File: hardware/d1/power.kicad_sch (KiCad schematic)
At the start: 46 parts, among them U10 BLM15PX601SN1D, U11 TPS7A2033PDBVR, U12 TPS7A2018PDBVR, U13 TPS7A2018PDBVR, U7 TPS7A2018PDBVR, U8 TPS7A2033PDBVR, U9 TPS560430XFDBVR

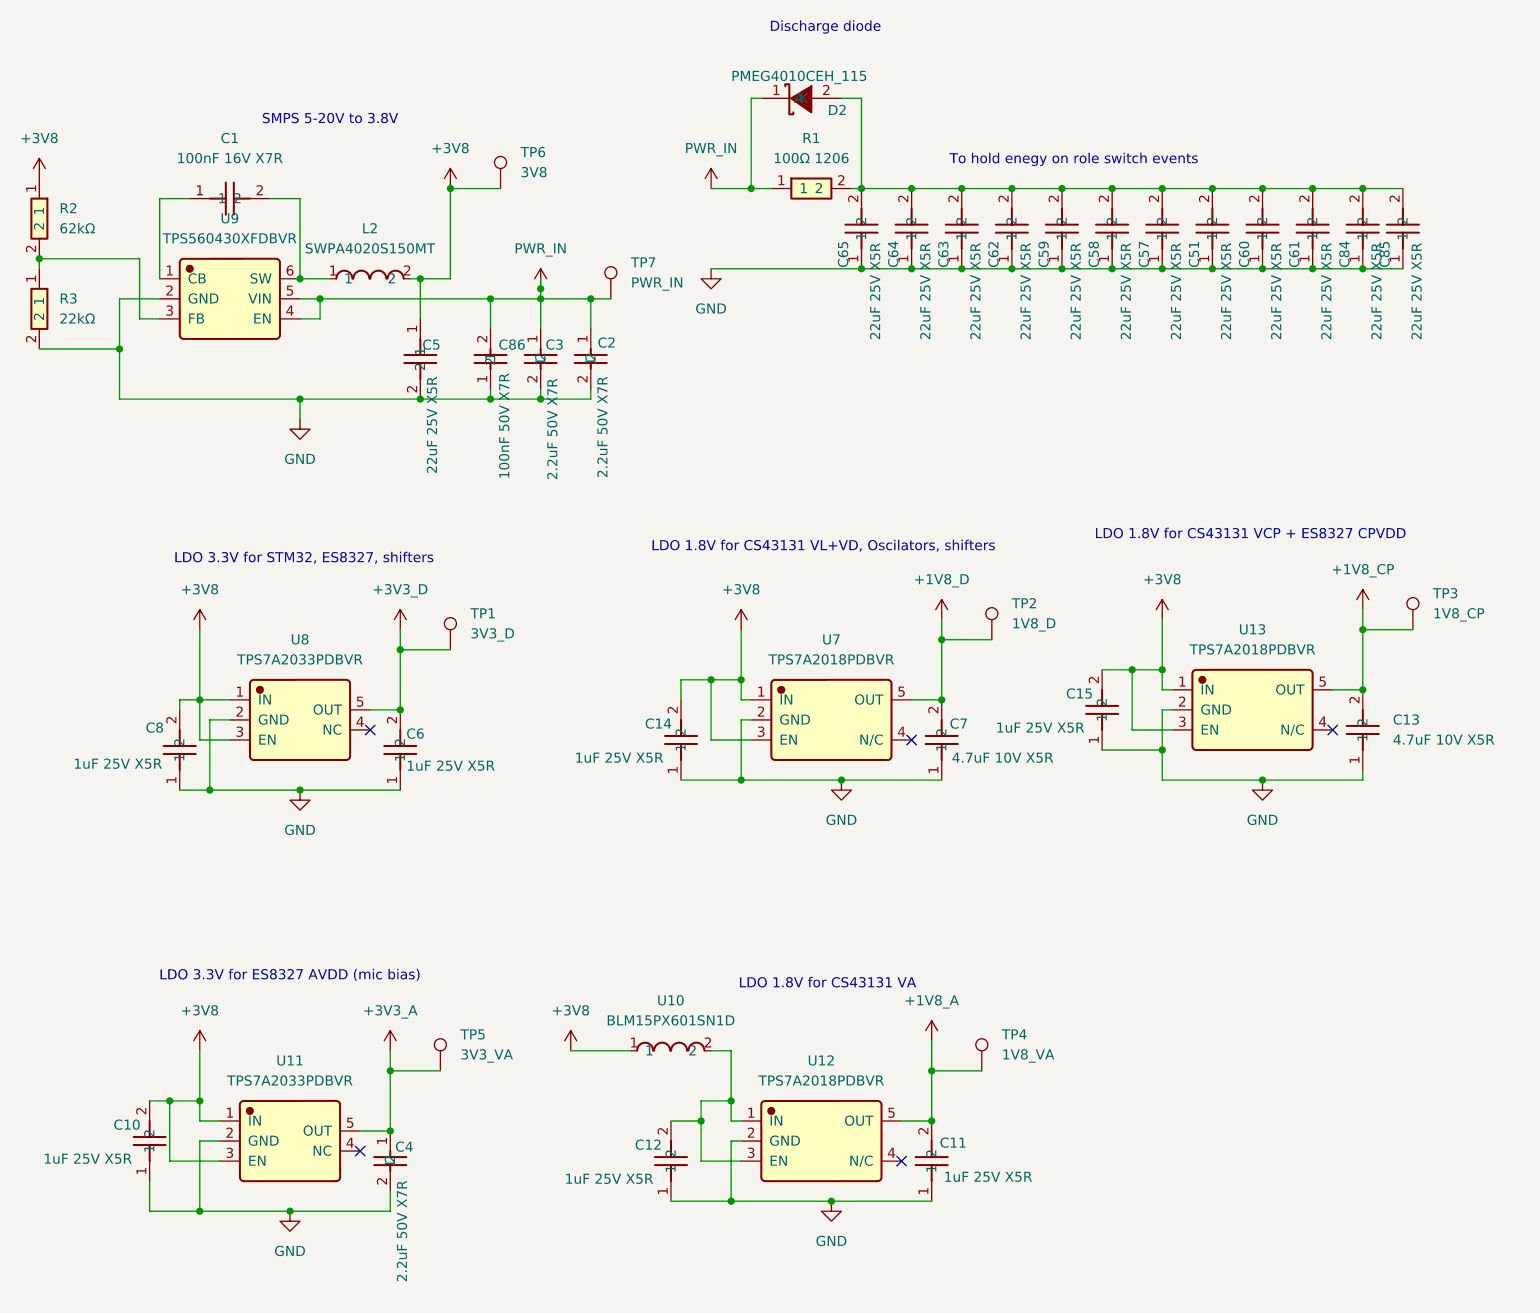
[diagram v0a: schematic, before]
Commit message: Fixes
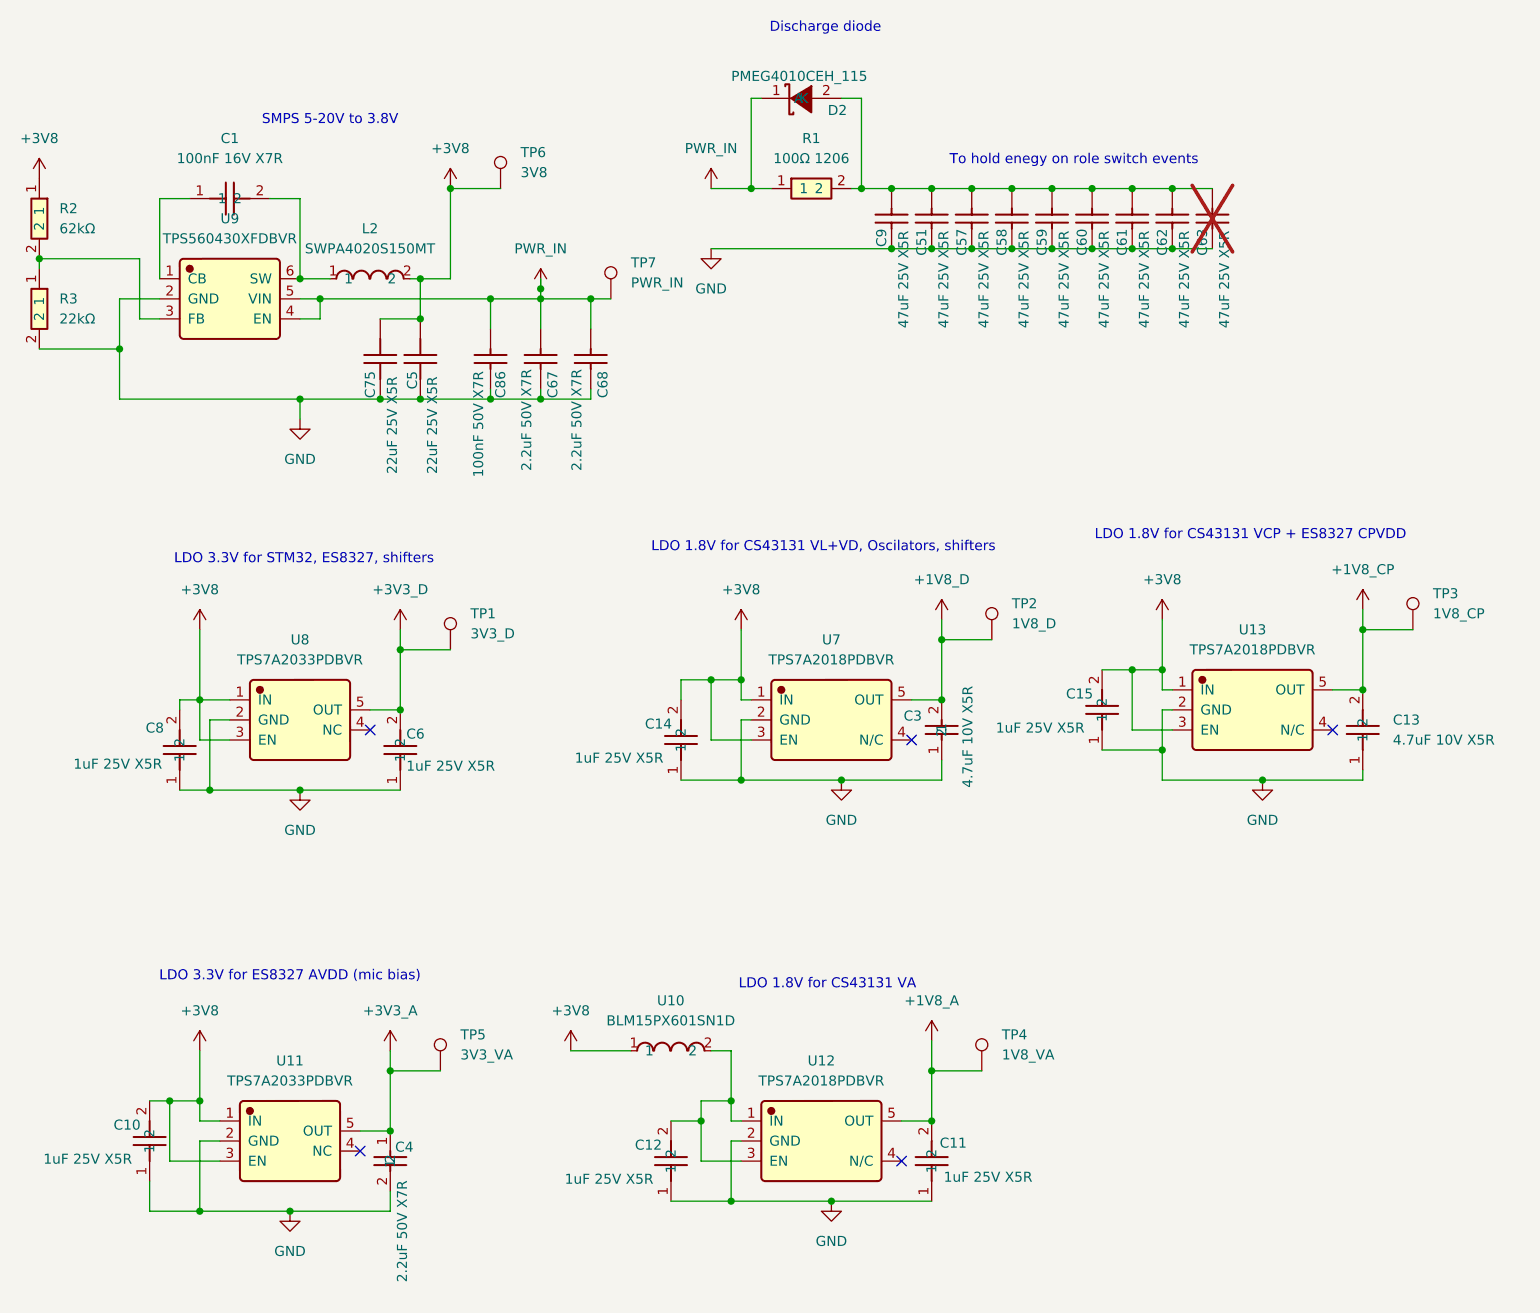
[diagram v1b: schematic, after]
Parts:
- removed C2, C3: 2.2uF 50V X7R, JLCImport:CC0805KKX7R9BB225, symbol JLCImport:CC0805KKX7R9BB225
- removed C51, C57, C58, C59, C60, C61, C62, C63, C64, C65, C84, C85: 22uF 25V X5R, JLCImport:CL21A226MAQNNNE, symbol JLCImport:CL21A226MAQNNNE
- removed C7: 4.7uF 10V X5R, JLCImport:CL05A475MP5NRNC, symbol JLCImport:CL05A475MP5NRNC
- added C3: 4.7uF 10V X5R, Capacitor_SMD:C_0603_1608Metric, symbol JLCImport:CL10A475KP8NNNC
- added C51, C57, C58, C59, C60, C61, C62, C63, C9: 47uF 25V X5R, Capacitor_SMD:C_1206_3216Metric, symbol JLCImport:C3216X5R1E476MTJ00E
- added C67, C68: 2.2uF 50V X7R, Capacitor_SMD:C_1206_3216Metric, symbol JLCImport:CL31B225KBHNNNE
- added C75: 22uF 25V X5R, JLCImport:CL21A226MAQNNNE, symbol JLCImport:CL21A226MAQNNNE
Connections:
- net +1V8_D: now also C3.2
- net +3V8: now also C75.1
- net GND: now also C3.1, C51.1, C57.1, C58.1, C59.1, C60.1, C61.1, C62.1, C63.1, C67.1, C68.1, C75.2, C9.1
- net PWR_IN: now also C67.2, C68.2
- net at D2.2 (A), R1.2: now also C51.2, C57.2, C58.2, C59.2, C60.2, C61.2, C62.2, C63.2, C9.2
